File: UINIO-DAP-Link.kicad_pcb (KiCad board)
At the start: 2 copper layers, 90.4 x 31 mm, 45 parts, among them J1 扩展板串口 & 电源输出, J2 扩展板 JTAG 输出, J3 JTAG_nTRST 跳线选择, J4 3.3V 跳线选择, J5 扩展板 SWD 输入, J6 DAPLink 固件下载接口, J7 JTAG/SWD 下载接口, U1 ME6211, U2 STM32F103C8T6, Y1 Crystal_GND24

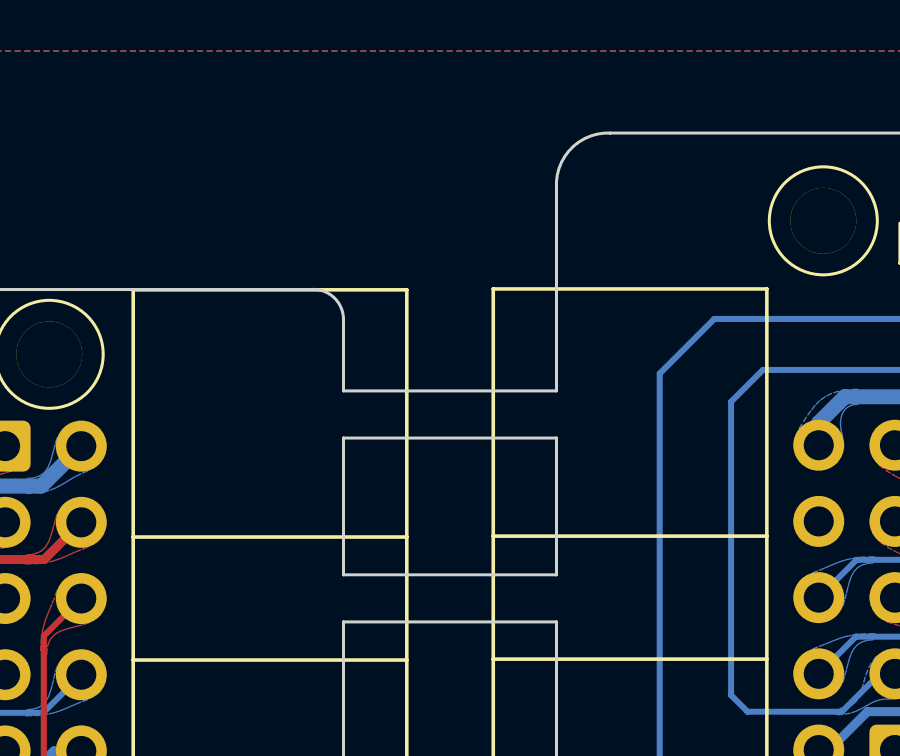
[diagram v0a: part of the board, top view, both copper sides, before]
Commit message: Release UINIO-DAP-Link 1.0.0.
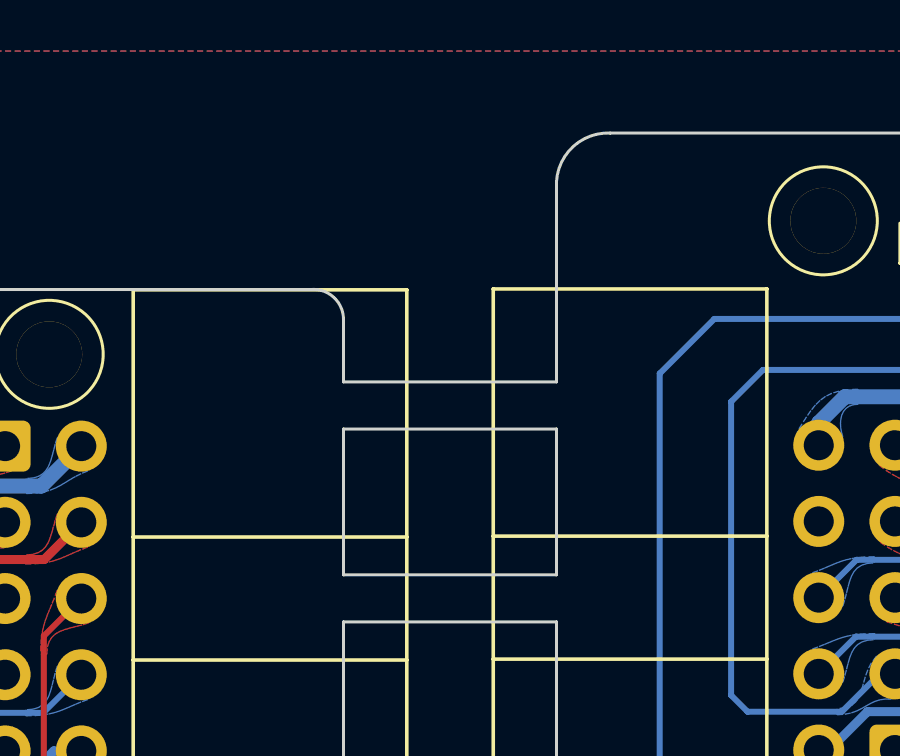
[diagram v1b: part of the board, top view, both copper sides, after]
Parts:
- moved ? 0.22 mm to (171.6, 107.2)
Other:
- outline, holes or cut-outs redrawn
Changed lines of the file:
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@@
   )
   (footprint "LOGO" (layer "B.Cu")
-    (at 171.34 107.17 -90)
+    (at 171.56 107.19 -90)
     (attr board_only exclude_from_pos_files exclude_from_bom)
     (fp_text reference "" (at 0 0 90) (layer "B.SilkS")
@@
   (gr_line (start 137.895 113.86) (end 142.945 113.86) (layer "B.SilkS") (width 0.1))
   (gr_line (start 188.92 92.874517) (end 188.92 121.774517) (layer "B.SilkS") (width 0.1))
-  (gr_line (start 144.52 102.05) (end 151.62 102.05) (layer "Edge.Cuts") (width 0.1))
+  (gr_line (start 144.52 101.75) (end 151.62 101.75) (layer "Edge.Cuts") (width 0.1))
   (gr_arc (start 102.68 98.06) (mid 102.987286 97.386407) (end 103.67 97.1) (layer "Edge.Cuts") (width 0.1))
   (gr_line (start 193.084 93.52) (end 193.084 121.27) (layer "Edge.Cuts") (width 0.1))
-  (gr_line (start 144.52 106.61) (end 144.52 102.05) (layer "Edge.Cuts") (width 0.1))
+  (gr_line (start 144.52 106.61) (end 144.52 101.75) (layer "Edge.Cuts") (width 0.1))
   (gr_line (start 103.67 117.7) (end 143.47 117.7) (layer "Edge.Cuts") (width 0.1))
   (gr_arc (start 143.42 97.1) (mid 144.195891 97.358999) (end 144.52 98.11) (layer "Edge.Cuts") (width 0.1))
-  (gr_line (start 151.62 100.48) (end 151.62 93.499) (layer "Edge.Cuts") (width 0.1))
+  (gr_line (start 151.62 100.18) (end 151.62 93.499) (layer "Edge.Cuts") (width 0.1))
   (gr_line (start 144.52 108.18) (end 151.62 108.18) (layer "Edge.Cuts") (width 0.1))
   (gr_arc (start 191.41 91.884) (mid 192.606648 92.33402) (end 193.084 93.52) (layer "Edge.Cuts") (width 0.1))
@@
   (gr_arc (start 193.084 121.27) (mid 192.531165 122.385345) (end 191.37 122.834) (layer "Edge.Cuts") (width 0.1))
   (gr_line (start 144.52 108.18) (end 144.52 113.05) (layer "Edge.Cuts") (width 0.1))
-  (gr_line (start 144.52 98.11) (end 144.52 100.48) (layer "Edge.Cuts") (width 0.1))
+  (gr_line (start 144.52 98.11) (end 144.52 100.18) (layer "Edge.Cuts") (width 0.1))
   (gr_line (start 153.41 91.884) (end 191.41 91.884) (layer "Edge.Cuts") (width 0.1))
   (gr_line (start 151.62 114.62) (end 151.62 121.249) (layer "Edge.Cuts") (width 0.1))
   (gr_arc (start 103.67 117.7) (mid 102.981443 117.426697) (end 102.68 116.75) (layer "Edge.Cuts") (width 0.1))
   (gr_line (start 151.62 113.05) (end 144.52 113.05) (layer "Edge.Cuts") (width 0.1))
-  (gr_line (start 144.52 100.48) (end 151.62 100.48) (layer "Edge.Cuts") (width 0.1))
+  (gr_line (start 144.52 100.18) (end 151.62 100.18) (layer "Edge.Cuts") (width 0.1))
   (gr_line (start 144.52 116.61) (end 144.52 114.62) (layer "Edge.Cuts") (width 0.1))
   (gr_line (start 103.67 97.1) (end 143.42 97.1) (layer "Edge.Cuts") (width 0.1))
@@
   (gr_line (start 102.68 98.06) (end 102.68 116.75) (layer "Edge.Cuts") (width 0.1))
   (gr_line (start 151.62 106.61) (end 144.52 106.61) (layer "Edge.Cuts") (width 0.1))
-  (gr_line (start 151.62 106.61) (end 151.62 102.05) (layer "Edge.Cuts") (width 0.1))
+  (gr_line (start 151.62 106.61) (end 151.62 101.75) (layer "Edge.Cuts") (width 0.1))
   (gr_arc (start 151.62 93.499) (mid 152.184916 92.325666) (end 153.41 91.884) (layer "Edge.Cuts") (width 0.1))
   (gr_line (start 144.52 98.11) (end 144.52 116.61) (layer "User.1") (width 0.1))
@@
   (gr_line (start 151.62 93.499) (end 151.62 121.249) (layer "User.1") (width 0.1))
   (gr_rect (start 102.68 97.1) (end 144.52 117.7) (layer "User.1") (width 0.1) (fill none))
+  (gr_rect (start 143.44 97.1) (end 146.88 100.18) (layer "User.1") (width 0.1) (fill none))
+  (gr_rect (start 144.58 114.62) (end 148.02 117.7) (layer "User.1") (width 0.1) (fill none))
   (gr_rect (start 149.26 113.05) (end 150.91 114.62) (layer "User.1") (width 0.1) (fill none))
   (gr_rect (start 151.62 91.88) (end 193.088 122.834) (layer "User.1") (width 0.1) (fill none))
